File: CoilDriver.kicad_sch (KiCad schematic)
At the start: 27 parts, among them Q1 IRLML2803, Q2 SiRA99DP, U2 DRV8235RTER

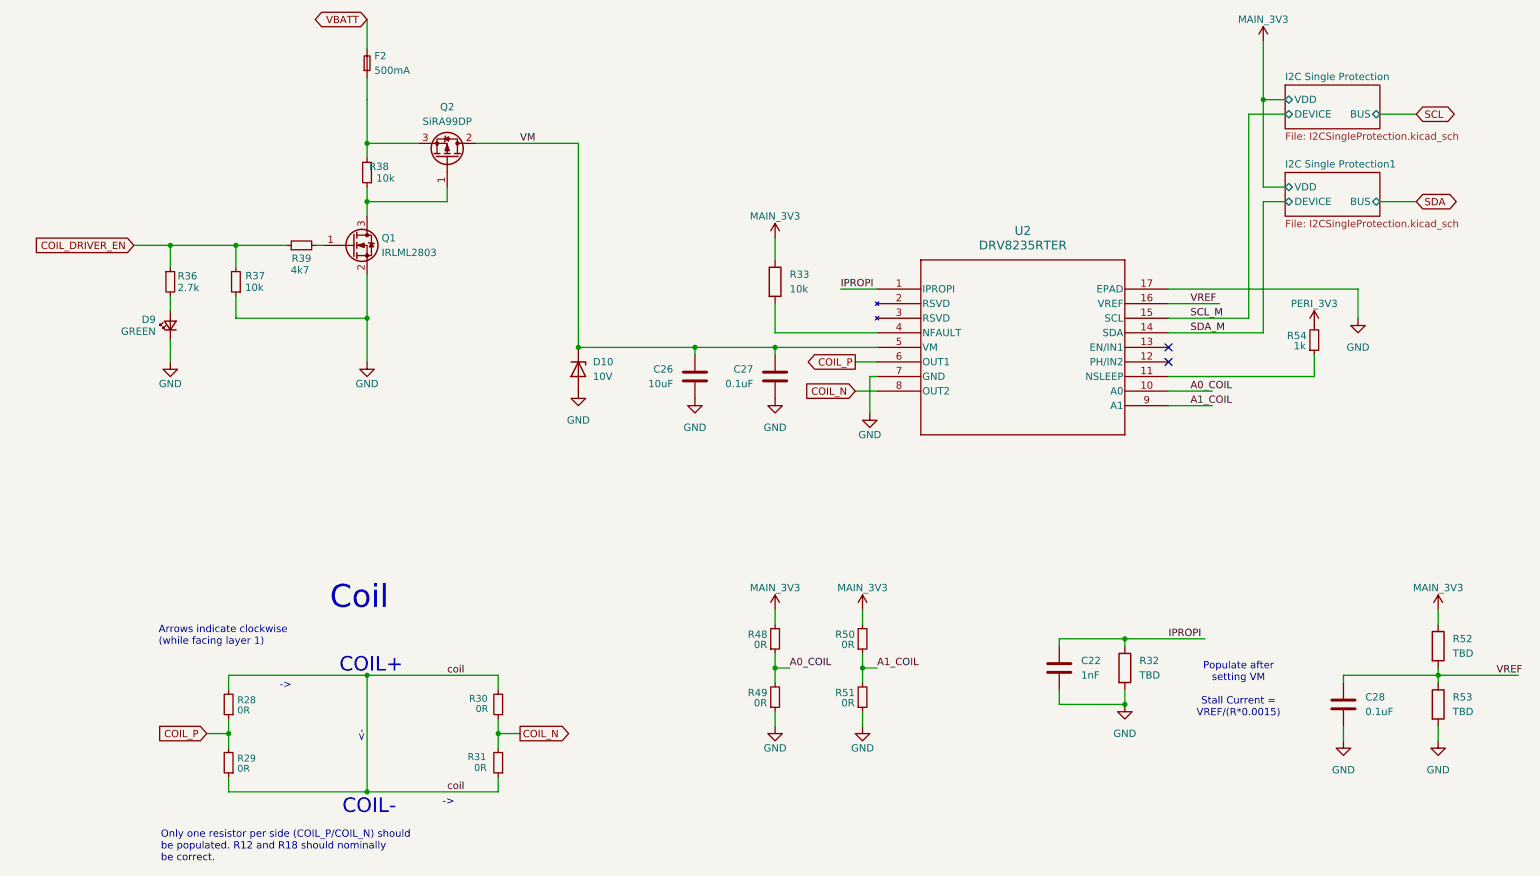
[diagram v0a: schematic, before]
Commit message: v3.1 Updates
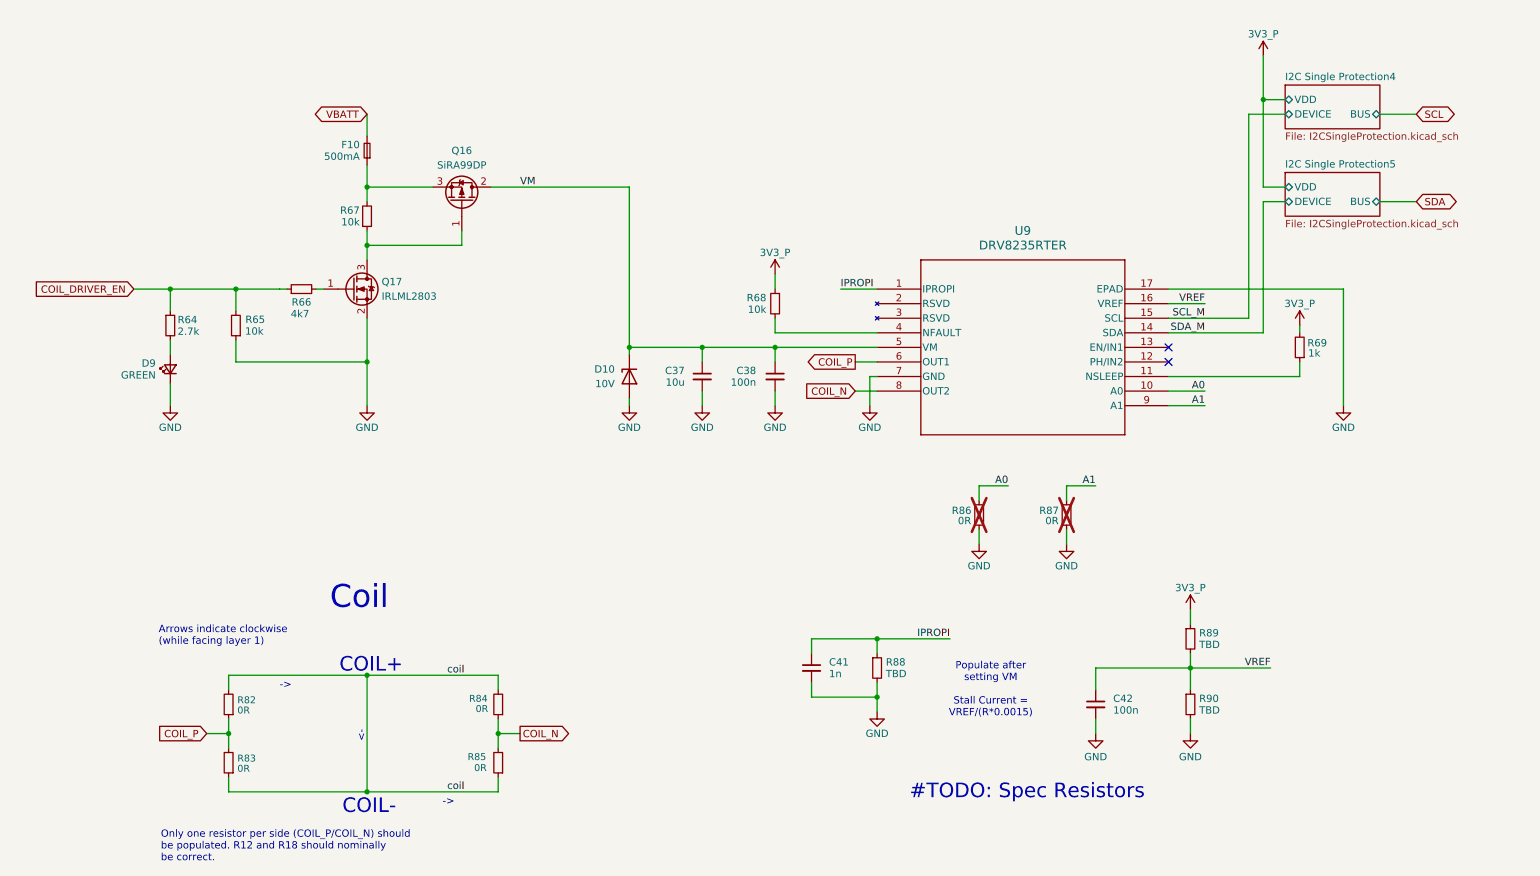
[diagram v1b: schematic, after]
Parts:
- removed R48, R50: 0R, Resistor_SMD:R_0603_1608Metric, symbol Device:R_Small
- C37: renamed from C26; value 10uF -> 10u; symbol Device:C -> Device:C_Small
- C38: renamed from C27; value 0.1uF -> 100n; symbol Device:C -> Device:C_Small
- C41: renamed from C22; value 1nF -> 1n; symbol Device:C -> Device:C_Small
- C42: renamed from C28; value 0.1uF -> 100n; symbol Device:C -> Device:C_Small
- R68: renamed from R33; symbol Device:R -> Device:R_Small
- R86: renamed from R49; now not fitted
- R87: renamed from R51; now not fitted
- R88: renamed from R32; symbol Device:R -> Device:R_Small
- R89: renamed from R52; symbol Device:R -> Device:R_Small
- R90: renamed from R53; symbol Device:R -> Device:R_Small
- renumbered F2 to F10, Q2 to Q16, Q1 to Q17, R36 to R64, R37 to R65, R39 to R66, R38 to R67, R54 to R69, R28 to R82, R29 to R83, R30 to R84, R31 to R85, U2 to U9
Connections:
- net PERI_3V3 is gone; now on net 3V3_P: R69.2
- net A0_COIL renamed A0
- net A1_COIL renamed A1
- net MAIN_3V3 renamed 3V3_P
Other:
- sheet I2C Single Protection renamed I2C Single Protection4
- sheet I2C Single Protection1 renamed I2C Single Protection5
- note added: "#TODO: Spec Resistors"
- company: (none) -> Carnegie Mellon University
- title: (none) -> Argus XY Solar Panel
- moved on the sheet: C37, C41, C42, D10, D9, F10, Q16, Q17, R64, R65, R66, R67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

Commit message: Local Stash
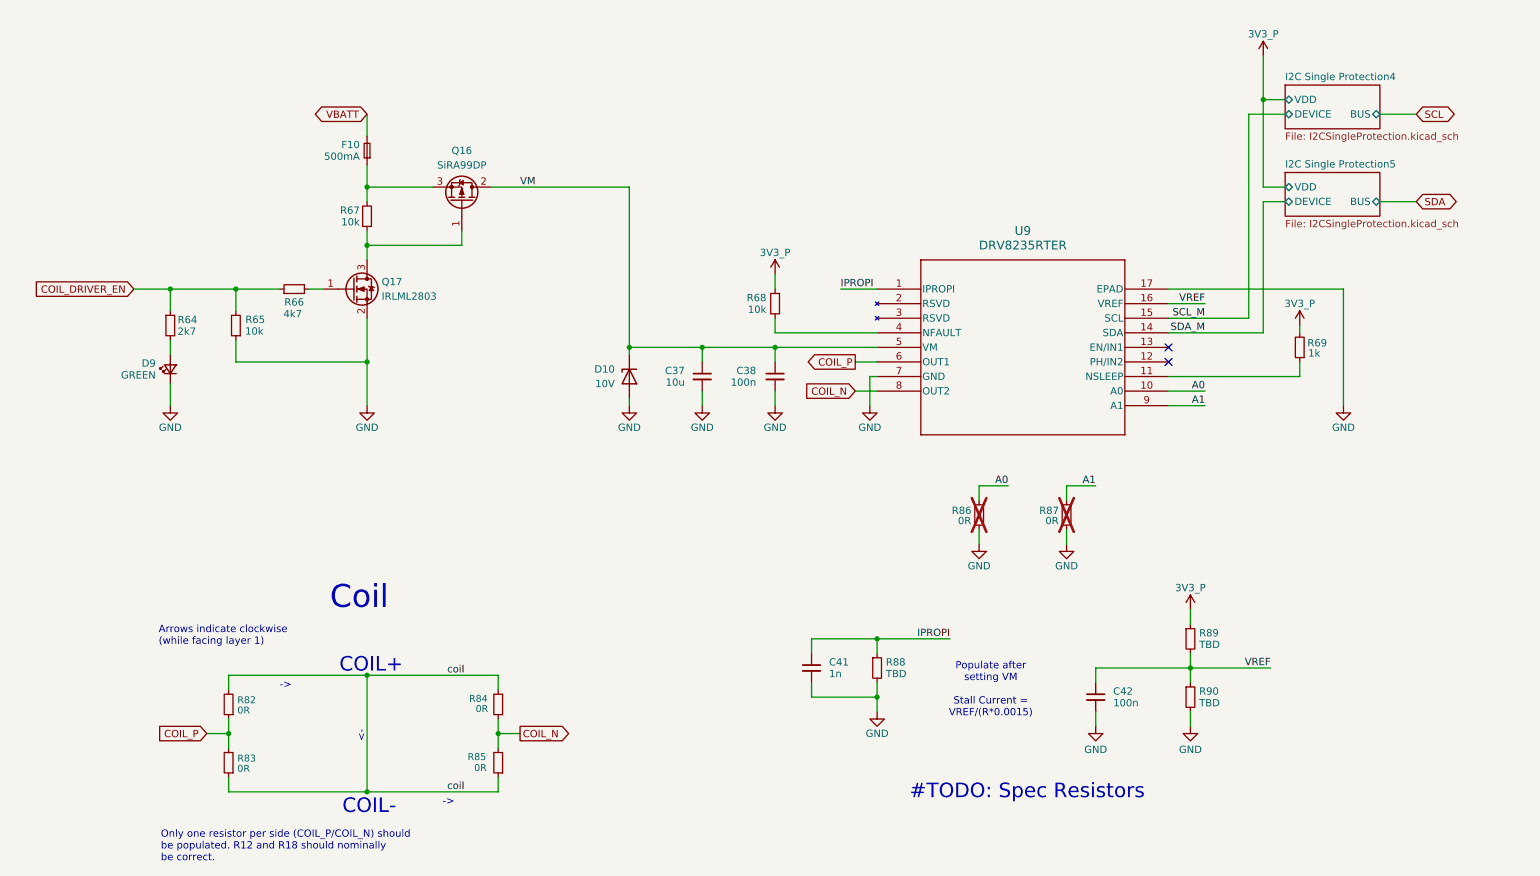
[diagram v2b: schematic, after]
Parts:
- R64: value 2.7k -> 2k7
- R69: symbol SolarPanels:R_Small -> Device:R_Small
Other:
- moved on the sheet: C42, R66, R90
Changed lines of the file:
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@@
 	(wire
 		(pts
-			(xy 205.74 137.16) (xy 205.74 140.97)
+			(xy 205.74 137.16) (xy 205.74 139.7)
 		)
 		(stroke
@@
 	(wire
 		(pts
-			(xy 222.25 146.05) (xy 222.25 148.59)
+			(xy 222.25 144.78) (xy 222.25 147.32)
 		)
 		(stroke
@@
 	(wire
 		(pts
-			(xy 69.85 71.12) (xy 71.12 71.12)
+			(xy 68.58 71.12) (xy 71.12 71.12)
 		)
 		(stroke
@@
 	(wire
 		(pts
-			(xy 222.25 137.16) (xy 222.25 140.97)
+			(xy 222.25 137.16) (xy 222.25 139.7)
 		)
 		(stroke
@@
 	(wire
 		(pts
-			(xy 205.74 146.05) (xy 205.74 148.59)
+			(xy 205.74 144.78) (xy 205.74 147.32)
 		)
 		(stroke
@@
 	(wire
 		(pts
-			(xy 63.5 71.12) (xy 64.77 71.12)
-		)
-		(stroke
-			(width 0)
-			(type default)
-		)
-	)
-	(wire
-		(pts
 			(xy 124.46 82.55) (xy 124.46 81.28)
 		)
@@
 	)
 	(symbol
-		(lib_name "R_Small_1")
 		(lib_id "Device:R_Small")
 		(at 222.25 132.08 0)
@@
 			)
 		)
-		(property "Value" "2.7k"
+		(property "Value" "2k7"
 			(at 45.72 79.248 0)
 			(effects
@@
 	(symbol
 		(lib_id "Device:C_Small")
-		(at 205.74 143.51 0)
+		(at 205.74 142.24 0)
 		(unit 1)
 		(exclude_from_sim no)
@@
 		(dnp no)
 		(property "Reference" "C42"
-			(at 208.788 142.494 0)
+			(at 208.788 141.224 0)
 			(effects
 				(font
@@
 		)
 		(property "Value" "100n"
-			(at 208.788 144.526 0)
+			(at 208.788 143.256 0)
 			(effects
 				(font
@@
 		)
 		(property "Footprint" "Capacitor_SMD:C_0603_1608Metric"
-			(at 205.74 143.51 0)
+			(at 205.74 142.24 0)
 			(effects
 				(font
@@
 		)
 		(property "Datasheet" "~"
-			(at 205.74 143.51 0)
+			(at 205.74 142.24 0)
 			(effects
 				(font
@@
 		)
 		(property "Description" "Unpolarized capacitor, small symbol"
-			(at 205.74 143.51 0)
+			(at 205.74 142.24 0)
 			(effects
 				(font
@@
 	(symbol
 		(lib_id "power:GND")
-		(at 205.74 148.59 0)
+		(at 205.74 147.32 0)
 		(unit 1)
 		(exclude_from_sim no)
@@
 		(dnp no)
 		(property "Reference" "#PWR036"
-			(at 205.74 154.94 0)
+			(at 205.74 153.67 0)
 			(effects
 				(font
@@
 		)
 		(property "Value" "GND"
-			(at 205.74 152.654 0)
+			(at 205.74 151.384 0)
 			(effects
 				(font
@@
 		)
 		(property "Footprint" ""
-			(at 205.74 148.59 0)
+			(at 205.74 147.32 0)
 			(effects
 				(font
@@
 		)
 		(property "Datasheet" ""
-			(at 205.74 148.59 0)
+			(at 205.74 147.32 0)
 			(effects
 				(font
@@
 		)
 		(property "Description" "Power symbol creates a global label with name \"GND\" , ground"
-			(at 205.74 148.59 0)
+			(at 205.74 147.32 0)
 			(effects
 				(font
@@
 	)
 	(symbol
-		(lib_id "SolarPanels:R_Small")
+		(lib_id "Device:R_Small")
 		(at 241.3 81.28 180)
 		(unit 1)
@@
 	)
 	(symbol
-		(lib_name "R_Small_2")
 		(lib_id "Device:R_Small")
 		(at 149.86 73.66 0)
@@
 	(symbol
 		(lib_id "Device:R_Small")
-		(at 67.31 71.12 90)
+		(at 66.04 71.12 90)
 		(unit 1)
 		(exclude_from_sim no)
@@
 		(dnp no)
 		(property "Reference" "R66"
-			(at 67.31 73.406 90)
+			(at 66.04 73.406 90)
 			(effects
 				(font
@@
 		)
 		(property "Value" "4k7"
-			(at 67.056 75.438 90)
+			(at 65.786 75.438 90)
 			(effects
 				(font
@@
 		)
 		(property "Footprint" "Resistor_SMD:R_0603_1608Metric"
-			(at 67.31 71.12 0)
+			(at 66.04 71.12 0)
 			(effects
 				(font
@@
 		)
 		(property "Datasheet" "~"
-			(at 67.31 71.12 0)
+			(at 66.04 71.12 0)
 			(effects
 				(font
@@
 		)
 		(property "Description" "Resistor, small symbol"
-			(at 67.31 71.12 0)
+			(at 66.04 71.12 0)
 			(effects
 				(font
@@
 			)
 		)
+		(property "Sim.Pin" "1=K 2=A"
+			(at 46.99 85.09 0)
+			(effects
+				(font
+					(size 1.27 1.27)
+				)
+				(hide yes)
+			)
+		)
 		(pin "2"
 		)
@@
 	(symbol
 		(lib_id "power:GND")
-		(at 222.25 148.59 0)
+		(at 222.25 147.32 0)
 		(unit 1)
 		(exclude_from_sim no)
@@
 		(dnp no)
 		(property "Reference" "#PWR039"
-			(at 222.25 154.94 0)
+			(at 222.25 153.67 0)
 			(effects
 				(font
@@
 		)
 		(property "Value" "GND"
-			(at 222.25 152.654 0)
+			(at 222.25 151.384 0)
 			(effects
 				(font
@@
 		)
 		(property "Footprint" ""
-			(at 222.25 148.59 0)
+			(at 222.25 147.32 0)
 			(effects
 				(font
@@
 		)
 		(property "Datasheet" ""
-			(at 222.25 148.59 0)
+			(at 222.25 147.32 0)
 			(effects
 				(font
@@
 		)
 		(property "Description" "Power symbol creates a global label with name \"GND\" , ground"
-			(at 222.25 148.59 0)
+			(at 222.25 147.32 0)
 			(effects
 				(font
@@
 	)
 	(symbol
-		(lib_name "R_Small_3")
 		(lib_id "Device:R_Small")
-		(at 222.25 143.51 0)
+		(at 222.25 142.24 0)
 		(unit 1)
 		(exclude_from_sim no)
@@
 		(dnp no)
 		(property "Reference" "R90"
-			(at 223.774 142.494 0)
+			(at 223.774 141.224 0)
 			(effects
 				(font
@@
 		)
 		(property "Value" "TBD"
-			(at 223.774 144.526 0)
+			(at 223.774 143.256 0)
 			(effects
 				(font
@@
 		)
 		(property "Footprint" "Resistor_SMD:R_0603_1608Metric"
-			(at 222.25 143.51 0)
+			(at 222.25 142.24 0)
 			(effects
 				(font
@@
 		)
 		(property "Datasheet" "~"
-			(at 222.25 143.51 0)
+			(at 222.25 142.24 0)
 			(effects
 				(font
@@
 		)
 		(property "Description" "Resistor, small symbol"
-			(at 222.25 143.51 0)
+			(at 222.25 142.24 0)
 			(effects
 				(font
@@
 	)
 	(symbol
-		(lib_name "R_Small_4")
 		(lib_id "Device:R_Small")
 		(at 167.64 137.16 0)
